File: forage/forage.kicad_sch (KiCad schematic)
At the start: 69 parts, among them J1 Conn_01x04_MountingPin, Q1 AO3400A, U1 STM32G431RBTx, U2 XC6206P332MR

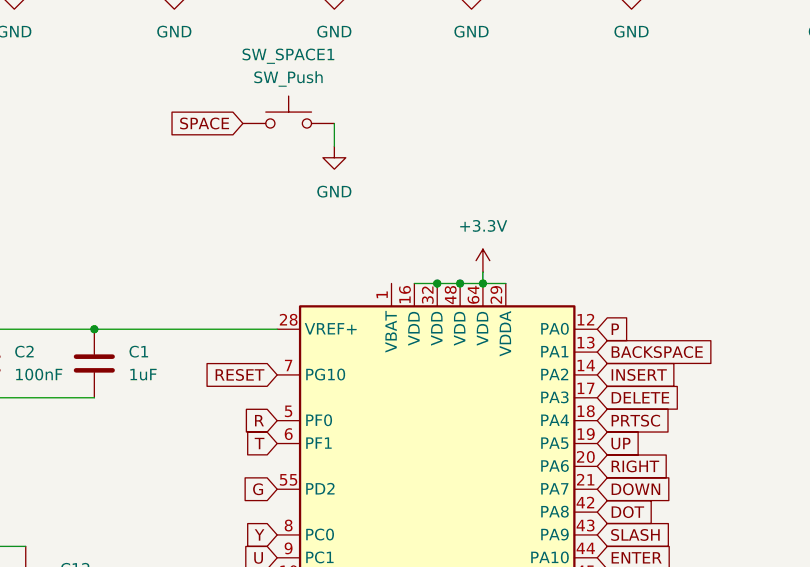
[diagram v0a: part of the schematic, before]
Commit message: connect vbat to the 3.3v net
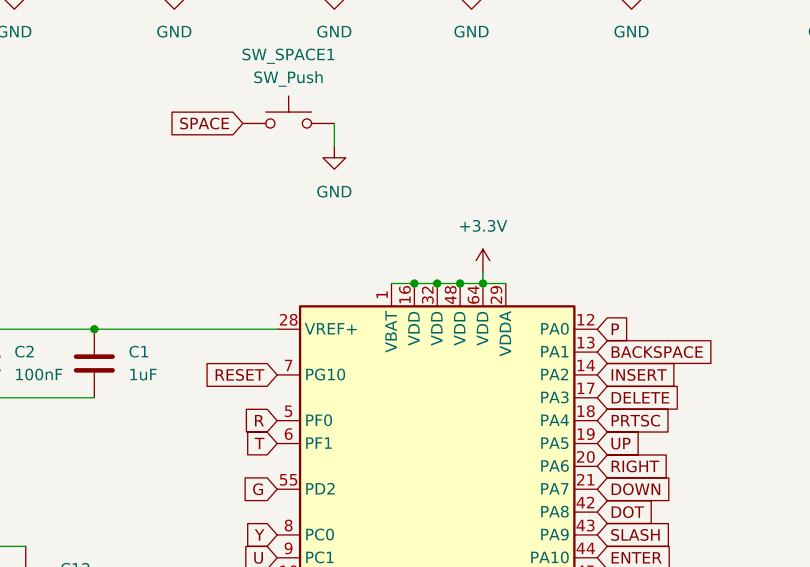
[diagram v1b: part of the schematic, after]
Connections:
- net +3.3V: now also U1.1 (VBAT)
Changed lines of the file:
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@@
+	)
+	(junction
+		(at 132.08 96.52)
+		(diameter 0)
+		(color 0 0 0 0)
 	)
 	(junction
@@
 		)
 		(stroke
+			(width 0)
+			(type default)
+		)
+	)
+	(wire
+		(pts
+			(xy 129.54 96.52) (xy 132.08 96.52)
+		)
+		(stroke

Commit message: recommended schmeccomended??? ok
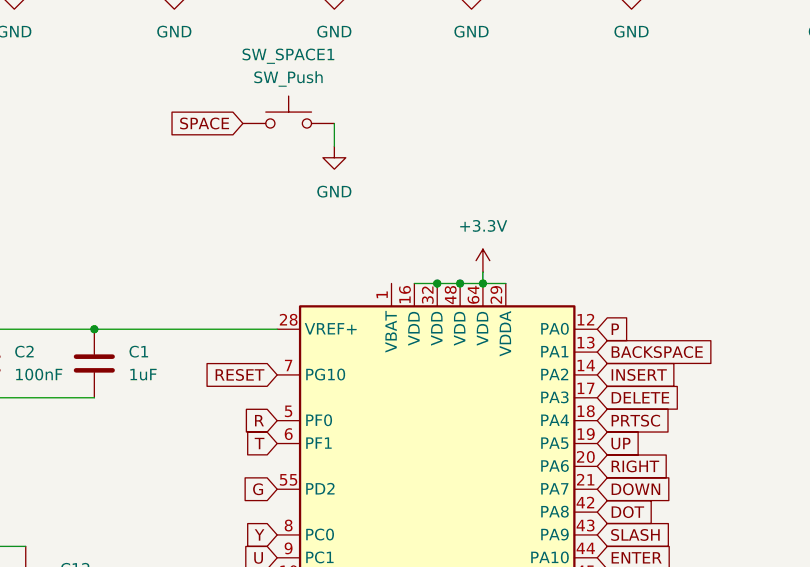
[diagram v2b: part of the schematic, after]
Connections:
- net +3.3V: no longer U1.1 (VBAT)
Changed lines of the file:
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@@
-	)
-	(junction
-		(at 132.08 96.52)
-		(diameter 0)
-		(color 0 0 0 0)
 	)
 	(junction
@@
 		)
 		(stroke
-			(width 0)
-			(type default)
-		)
-	)
-	(wire
-		(pts
-			(xy 129.54 96.52) (xy 132.08 96.52)
-		)
-		(stroke
